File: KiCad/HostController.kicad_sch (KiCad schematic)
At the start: 4 parts, among them U301 STM32G0B1KCTx, Y301 Crystal_Small

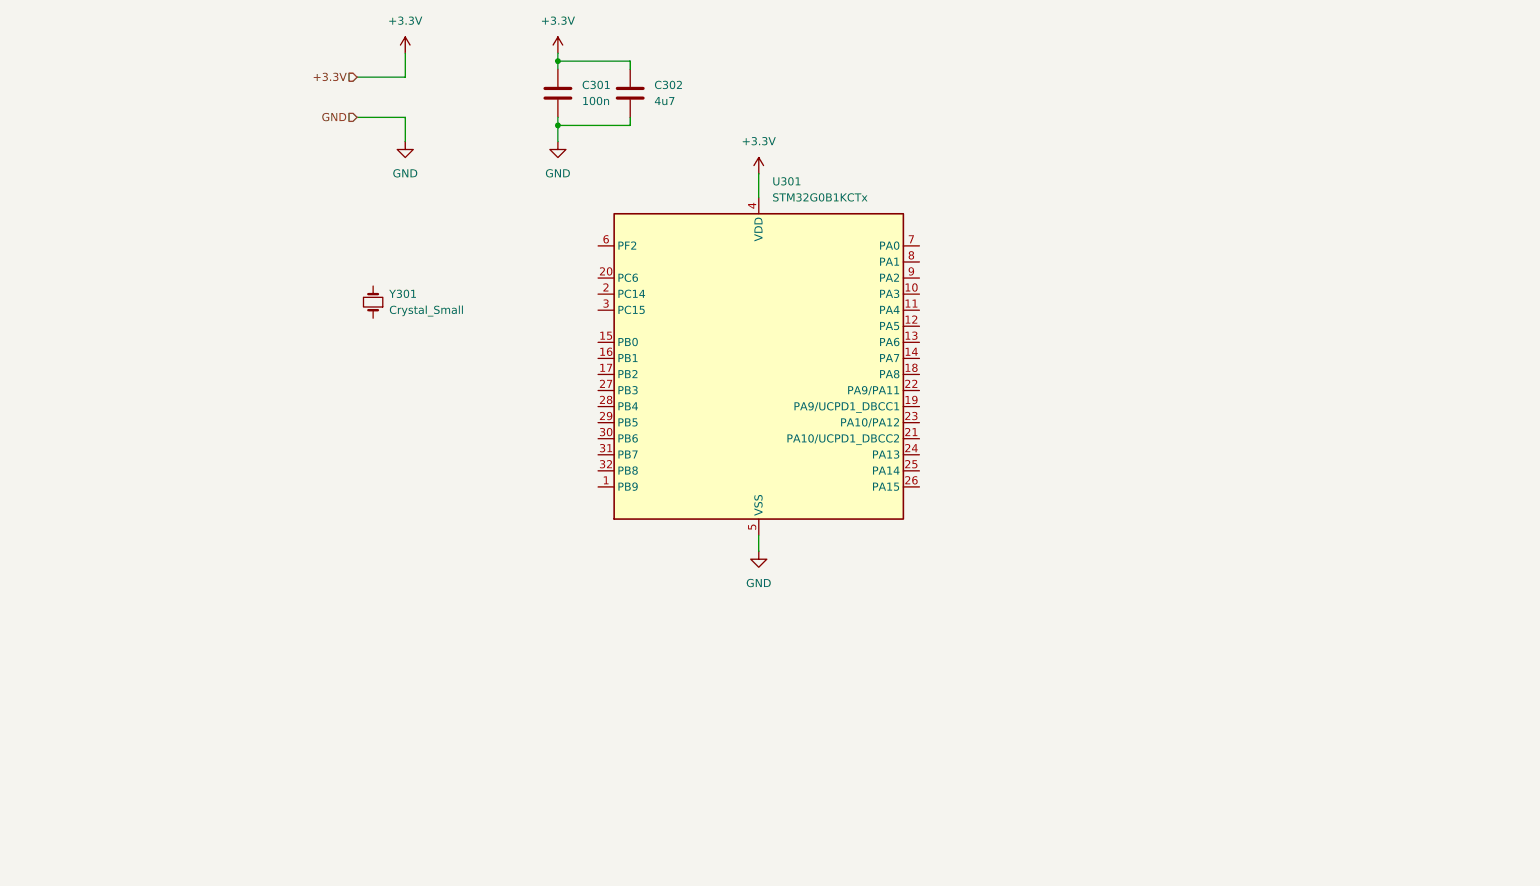
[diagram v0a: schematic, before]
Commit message: work
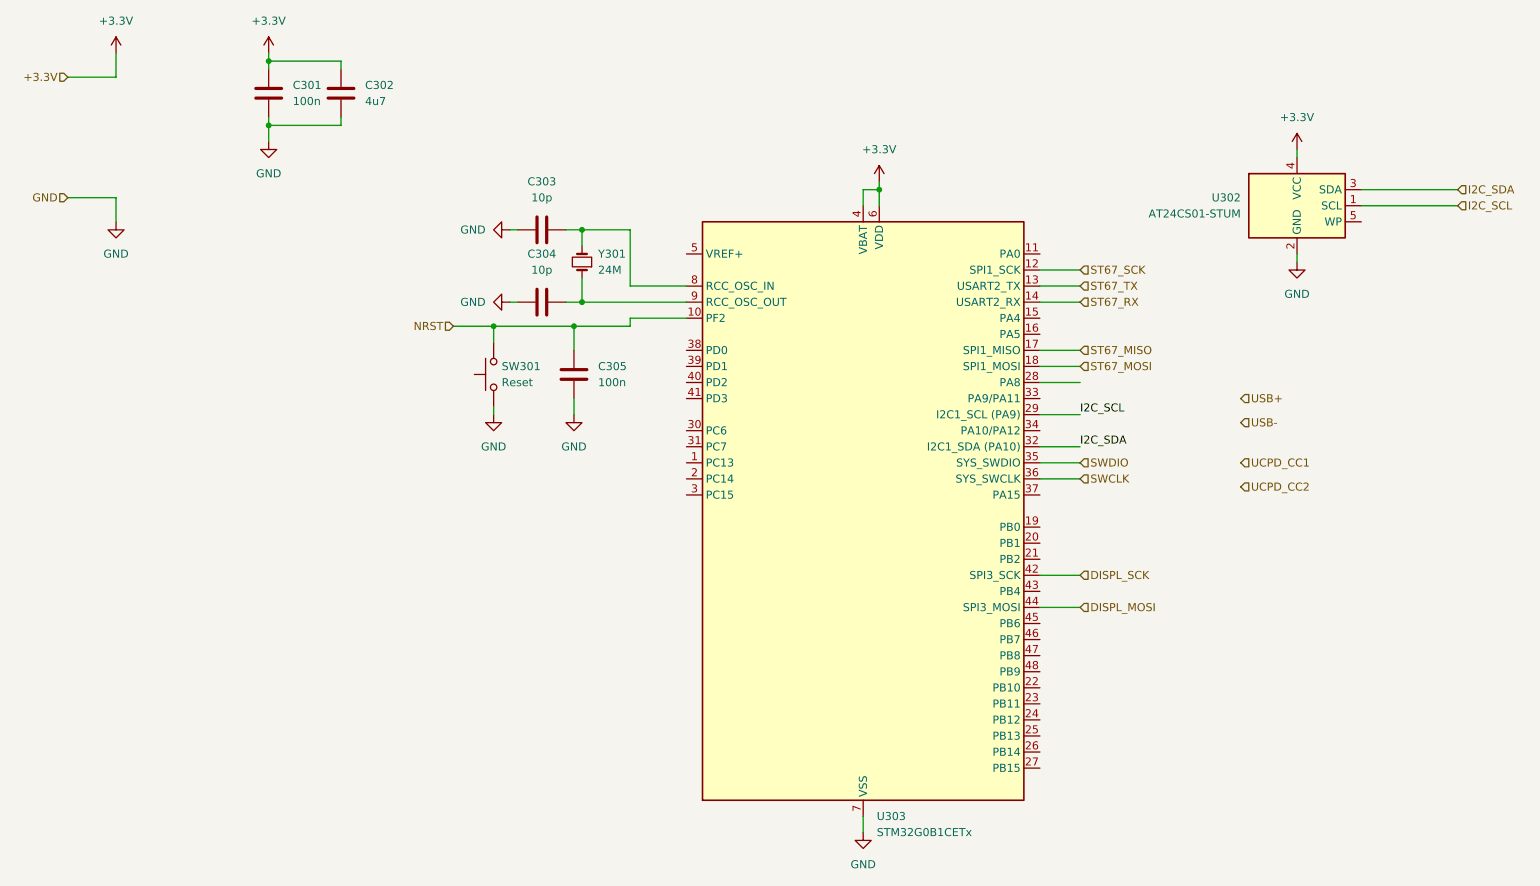
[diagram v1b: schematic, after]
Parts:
- removed U301: STM32G0B1KCTx, Package_QFP:LQFP-32_7x7mm_P0.8mm, symbol MCU_ST_STM32G0:STM32G0B1KCTx
- added C303, C304: 10p, Capacitor_SMD:C_0603_1608Metric, symbol Device:C
- added C305: 100n, Capacitor_SMD:C_0603_1608Metric, symbol Device:C
- added SW301: Reset, symbol Switch:SW_Push
- added U302: AT24CS01-STUM, Package_TO_SOT_SMD:SOT-23-5, symbol Memory_EEPROM:AT24CS01-STUM
- added U303: STM32G0B1CETx, Package_QFP:LQFP-48_7x7mm_P0.5mm, symbol MCU_ST_STM32G0:STM32G0B1CETx
- Y301: value Crystal_Small -> 24M
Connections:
- net +3.3V: now also U302.4 (VCC), U303.4 (VBAT), U303.6 (VDD)
- net GND: now also C303.1, C304.1, C305.2, SW301.1, U302.2 (GND), U303.7 (VSS)
- net at Y301.1: now also C304.2, U303.9 (PF1)
- net at Y301.2: now also C303.2, U303.8 (PF0)
- new net DISPL_MOSI: U303.44 (PB5)
- new net DISPL_SCK: U303.42 (PB3)
- new net I2C_SCL: U302.1 (SCL), U303.29 (PA9/UCPD1_DBCC1)
- new net I2C_SDA: U302.3 (SDA), U303.32 (PA10/UCPD1_DBCC2)
- new net NRST: C305.1, SW301.2, U303.10 (PF2)
- new net ST67_MISO: U303.17 (PA6)
- new net ST67_MOSI: U303.18 (PA7)
- new net ST67_RX: U303.14 (PA3)
- new net ST67_SCK: U303.12 (PA1)
- new net ST67_TX: U303.13 (PA2)
- new net SWCLK: U303.36 (PA14)
- new net SWDIO: U303.35 (PA13)
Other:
- moved on the sheet: C301, C302, Y301
